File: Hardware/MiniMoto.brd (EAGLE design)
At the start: 25.4 x 25.4 mm, 23 parts, among them J1 M02PTH3, J2 M023.5MM, J3 M02PTH3, J4 M023.5MM, J5 M02PTH3, J6 M023.5MM, J7 M04X2, U1 DRV8830

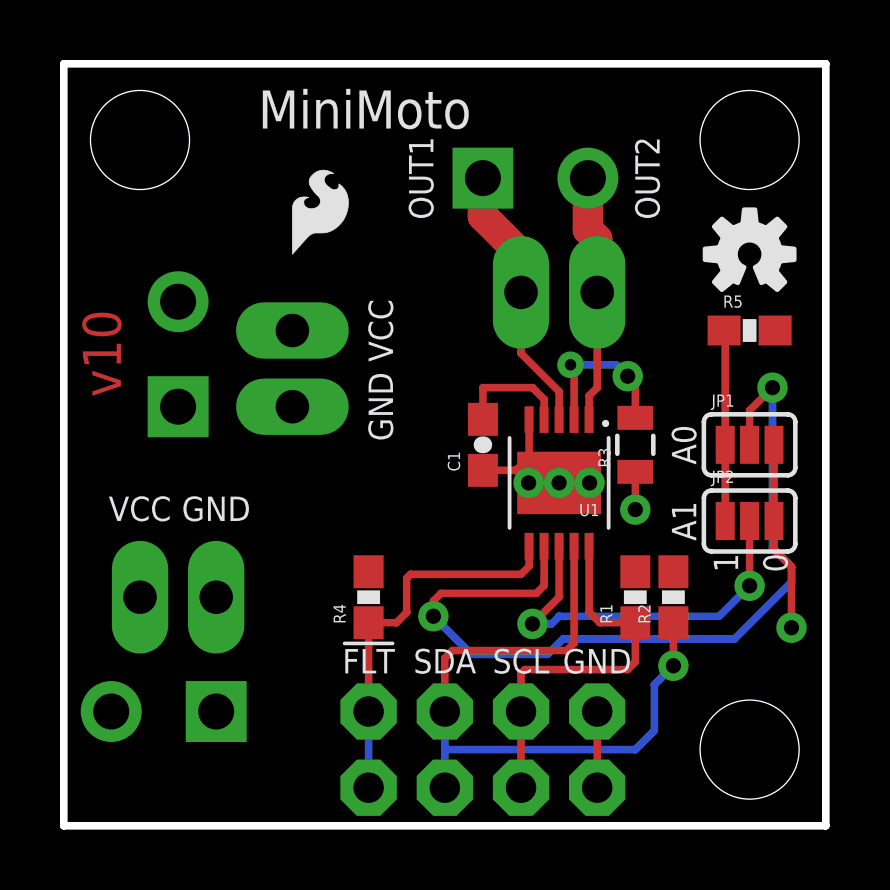
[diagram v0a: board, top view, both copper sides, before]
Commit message: Updated to v10 for release
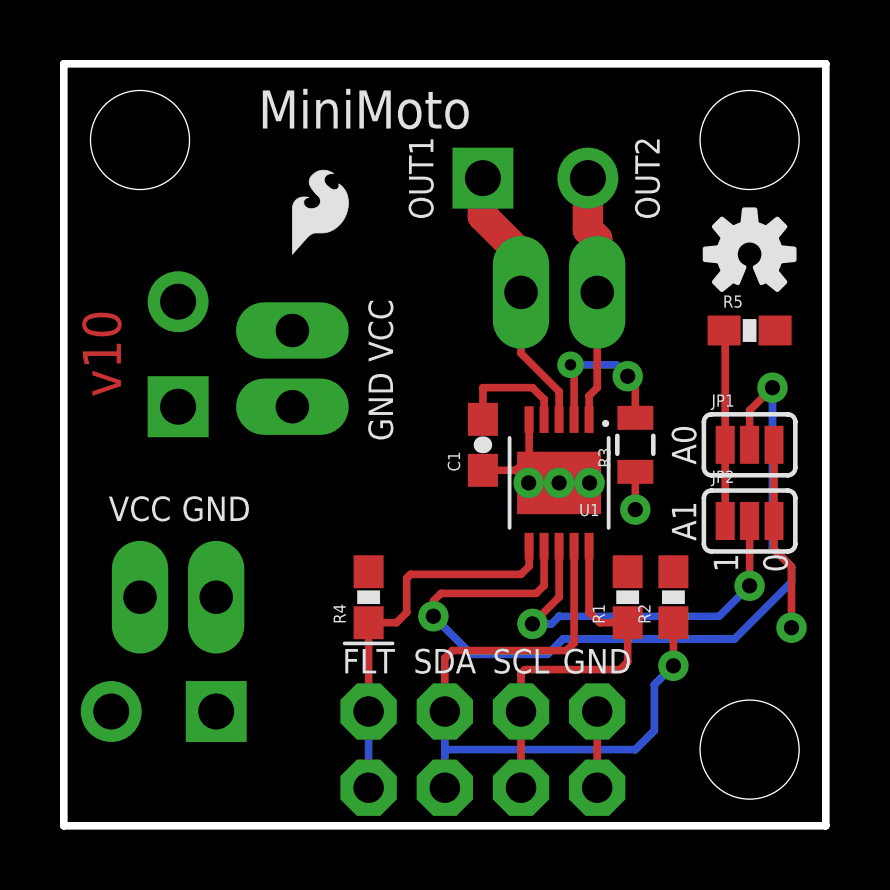
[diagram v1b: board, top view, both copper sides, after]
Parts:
- moved R1 0.25 mm to (18.8, 7.62)
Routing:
- net SCL: track 13.0 -> 12.5 mm
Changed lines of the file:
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@@
 <?xml version="1.0" encoding="utf-8"?>
 <!DOCTYPE eagle SYSTEM "eagle.dtd">
-<eagle version="6.4">
+<eagle version="6.3">
 <drawing>
 <settings>
@@
 <elements>
 <element name="FRAME1" library="SparkFun-Aesthetics" package="CREATIVE_COMMONS" value="FRAME-LETTER" x="-77.47" y="11.43"/>
-<element name="R1" library="SparkFun-Resistors" package="0603-RES" value="1K" x="19.05" y="7.62" rot="R90">
-<attribute name="PROD_ID" value="RES-07856" x="48.26" y="50.8" size="1.778" layer="27" rot="R90" display="off"/>
+<element name="R1" library="SparkFun-Resistors" package="0603-RES" value="1K" x="18.796" y="7.62" rot="R90">
+<attribute name="PROD_ID" value="RES-07856" x="48.006" y="50.8" size="1.778" layer="27" rot="R90" display="off"/>
 </element>
 <element name="R2" library="SparkFun-Resistors" package="0603-RES" value="1K" x="20.32" y="7.62" rot="R90">
@@
 <contactref element="J7" pad="5"/>
 <contactref element="J7" pad="6"/>
-<wire x1="19.05" y1="6.77" x2="19.05" y2="5.461" width="0.254" layer="1"/>
-<wire x1="19.05" y1="5.461" x2="18.796" y2="5.207" width="0.254" layer="1"/>
-<wire x1="18.796" y1="5.207" x2="15.367" y2="5.207" width="0.254" layer="1"/>
+<wire x1="18.796" y1="6.77" x2="18.796" y2="5.461" width="0.254" layer="1"/>
+<wire x1="18.796" y1="5.461" x2="18.542" y2="5.207" width="0.254" layer="1"/>
+<wire x1="18.542" y1="5.207" x2="15.367" y2="5.207" width="0.254" layer="1"/>
 <wire x1="15.367" y1="5.207" x2="15.24" y2="5.08" width="0.254" layer="1"/>
 <wire x1="17.51" y1="9.3205" x2="17.51" y2="7.128" width="0.254" layer="1"/>
 <wire x1="17.51" y1="7.128" x2="17.868" y2="6.77" width="0.254" layer="1"/>
-<wire x1="19.05" y1="6.77" x2="17.868" y2="6.77" width="0.254" layer="1"/>
+<wire x1="18.796" y1="6.77" x2="17.868" y2="6.77" width="0.254" layer="1"/>
 <wire x1="15.24" y1="5.08" x2="15.24" y2="3.81" width="0.254" layer="1"/>
 <wire x1="15.24" y1="3.81" x2="15.24" y2="1.27" width="0.254" layer="1"/>
